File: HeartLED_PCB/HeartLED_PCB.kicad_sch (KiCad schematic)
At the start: 35 parts, among them U1 ICM7555IBAZ-T, U2 CD4017BM96, U3 TPS61222DCKR, U4 HX SS12F44G4

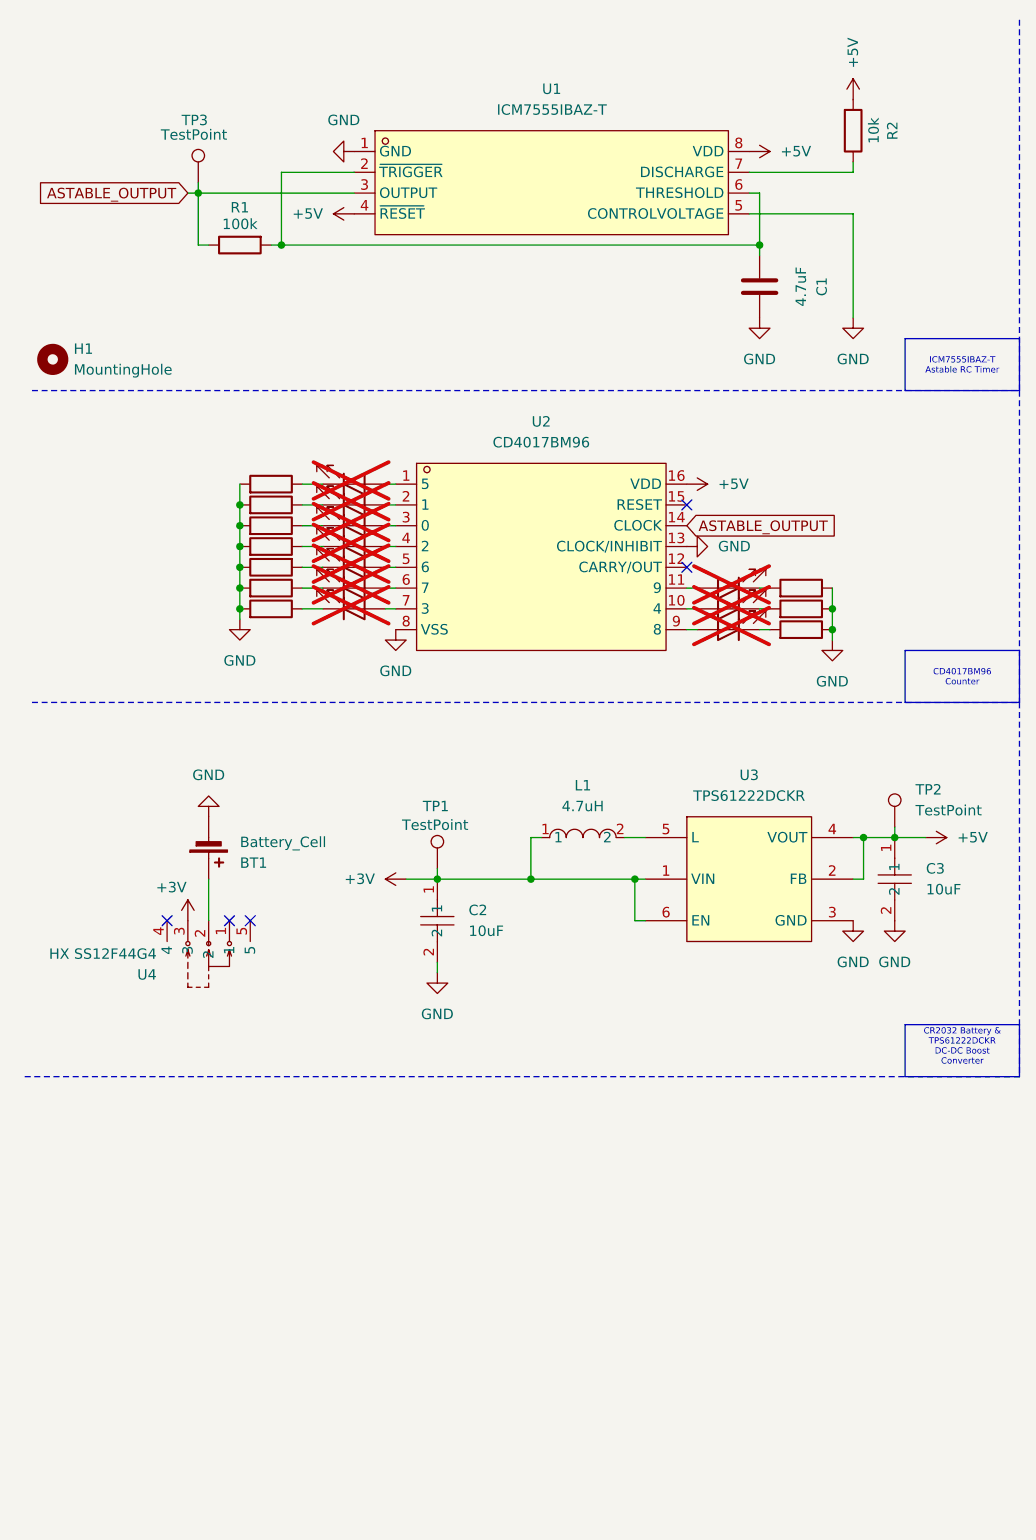
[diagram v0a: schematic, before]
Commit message: Ready to route
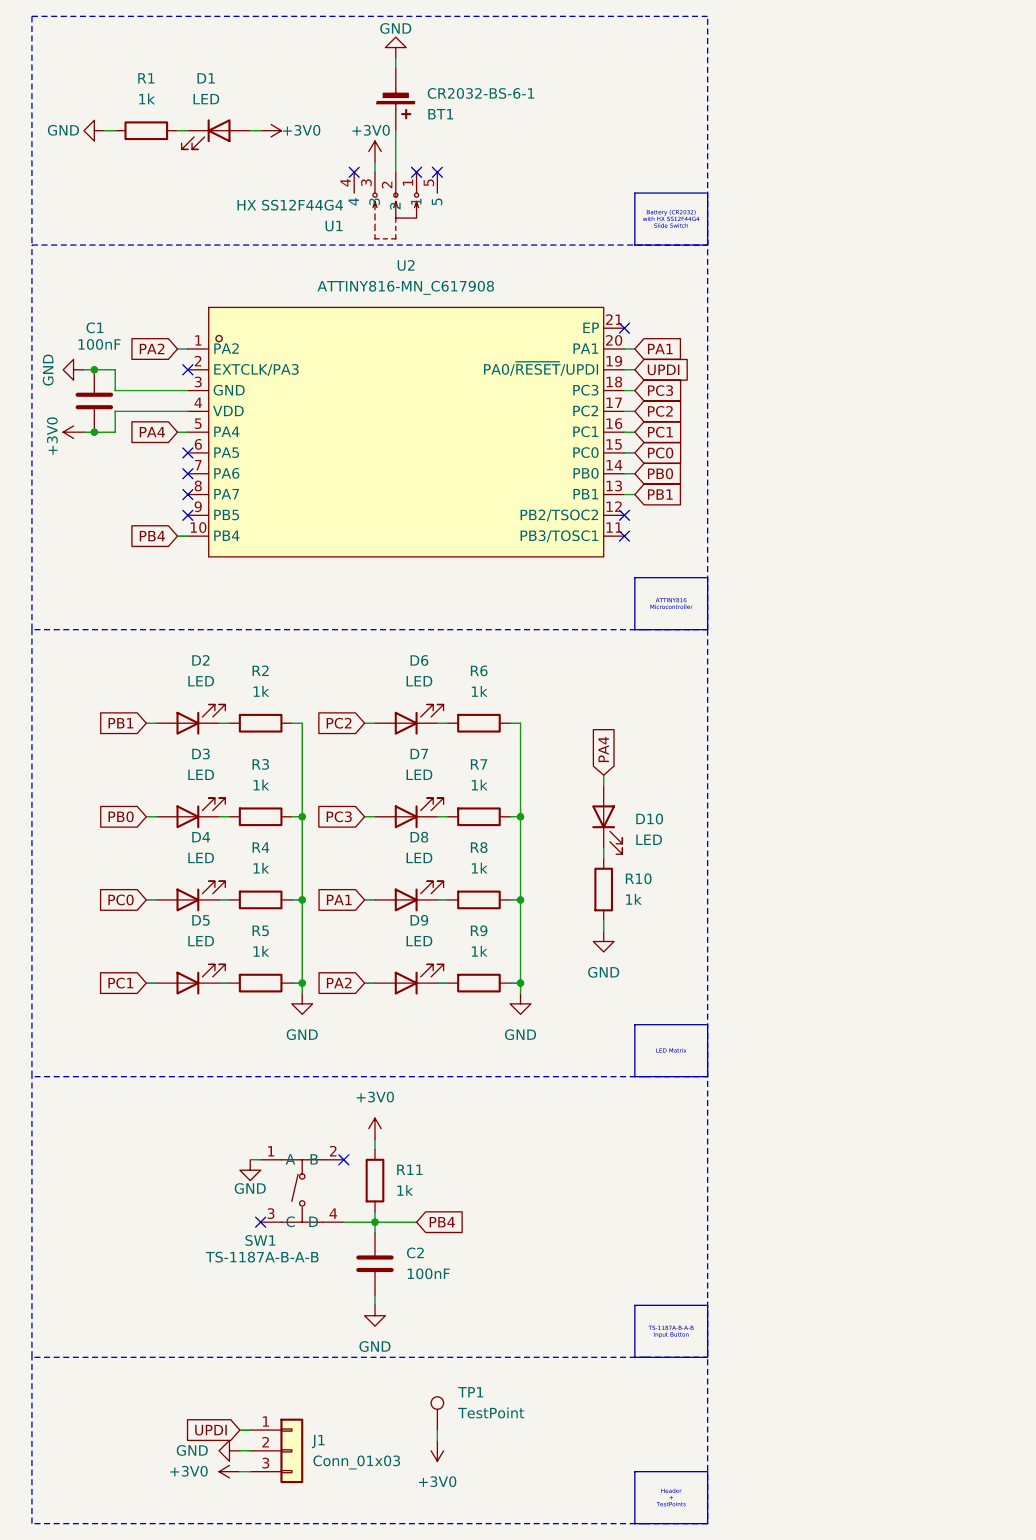
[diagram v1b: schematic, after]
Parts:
- removed C2, C3: 10uF, FOOTPRINTS:CL10A106MQ8NNNC, symbol CL10A106MQ8NNNC:CL10A106MQ8NNNC
- removed H1: MountingHole, MountingHole:MountingHole_2.1mm, symbol Mechanical:MountingHole
- removed L1: 4.7uH, FOOTPRINTS:LQH3NPN4R7MMEL, symbol LQH3NPN4R7MMEL:LQH3NPN4R7MMEL
- removed R12: 3.3k, FOOTPRINTS:0402WGJ0332TCE, symbol Device:R
- removed TP2, TP3: TestPoint, TestPoint:TestPoint_Pad_D1.0mm, symbol Connector:TestPoint
- removed U1: ICM7555IBAZ-T, FOOTPRINTS:ICM7555IBAZ-T, symbol ICM7555IBAZ-T:ICM7555IBAZ-T
- removed U2: CD4017BM96, FOOTPRINTS:CD4017BM96, symbol CD4017BM96:CD4017BM96
- removed U3: TPS61222DCKR, FOOTPRINTS:TPS61222DCKR, symbol TPS61222DCKR:TPS61222DCKR
- added C2: 100nF, FOOTPRINTS:0201X104K100CT, symbol Device:C
- added J1: Conn_01x03, Connector_PinHeader_2.54mm:PinHeader_1x03_P2.54mm_Vertical, symbol Connector_Generic:Conn_01x03
- added SW1: TS-1187A-B-A-B, FOOTPRINTS:TS-1187A-B-A-B, symbol TS-1187A-B-A-B:TS-1187A-B-A-B
- added U2: ATTINY816-MN_C617908, FOOTPRINTS:ATTINY816-MN, symbol ATTINY816-MN:ATTINY816-MN_C617908
- BT1: value Battery_Cell -> CR2032-BS-6-1; footprint Battery:BatteryHolder_Keystone_1060_1x2032 -> FOOTPRINTS:CR2032-BS-6-1; LCSC C5370859 -> C70377
- C1: value 4.7uF -> 100nF; footprint FOOTPRINTS:CL10A475KP8NNNC -> FOOTPRINTS:0201X104K100CT; LCSC C1705 -> C301918
- D1: footprint LED_THT:LED_D3.0mm -> FOOTPRINTS:F.0603.00026_P2-0603B1TS2-06T-001; LCSC (none) -> C7496819; now fitted
- D10, D2, D3, D4, D5, D6, D7, D8, D9: footprint LED_THT:LED_D3.0mm -> FOOTPRINTS:F.0603.00139_P2-0603R1TS2-06T-002; LCSC (none) -> C7496820; now fitted
- R1: value 100k -> 1k; footprint FOOTPRINTS:0603WAJ0104T5E -> FOOTPRINTS:0402WGJ0102TCE; LCSC C15458 -> C25543
- R10, R11, R3, R4, R5, R6, R7, R8, R9: value 3.3k -> 1k; footprint FOOTPRINTS:0402WGJ0332TCE -> FOOTPRINTS:0402WGJ0102TCE; LCSC C25936 -> C25543
- R2: value 10k -> 1k; footprint FOOTPRINTS:0402WGJ0103TCE -> FOOTPRINTS:0402WGJ0102TCE; LCSC C25531 -> C25543
- TP1: footprint TestPoint:TestPoint_Pad_D1.0mm -> TestPoint:TestPoint_Pad_D1.5mm
- renumbered U4 to U1
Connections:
- net +3V is gone; now on net +3V0: TP1.1, U1.3
- net +5V is gone; now on an unnamed net: R2.2
- net ASTABLE_OUTPUT is gone; now on net GND: R1.1
- net GND: now also C1.1, R10.2, R2.1, R3.1, R4.1, R5.1, R6.1, R8.1, R9.1, C2.2, J1.2 (Pin_2), SW1.1 (A), U2.3 (GND); no longer C1.2, R10.1, R11.1, R3.2, R4.2, R5.2, R6.2, R8.2, R9.2
- net +3V0: now reaches D1.2 (A)
- net +3V0: now also C1.2, R11.1, J1.3 (Pin_3), U2.4 (VDD)
- net PA2: now reaches D9.2 (A)
- net PA2: now also U2.1 (PA2)
- net PA4: now reaches D10.2 (A)
- net PA4: now also U2.5 (PA4)
- net PB1: now reaches D2.2 (A)
- net PB1: now also U2.13 (PB1)
- net PB0: now reaches D3.2 (A)
- net PB0: now also U2.14 (PB0)
- net PC0: now reaches D4.2 (A)
- net PC0: now also U2.15 (PC0)
- net PC1: now reaches D5.2 (A)
- net PC1: now also U2.16 (PC1)
- net PC2: now reaches D6.2 (A)
- net PC2: now also U2.17 (PC2)
- net PC3: now reaches D7.2 (A)
- net PC3: now also U2.18 (PC3)
- net PA1: now reaches D8.2 (A)
- net PA1: now also U2.20 (PA1)
- net at D6.1 (K): now also R6.2; no longer R8.1
- net at D1.1 (K): now also R1.2; no longer R3.1
- net at D8.1 (K): now also R8.2; no longer R10.2
- net at D3.1 (K): now also R3.2; no longer R5.1
- net at D10.1 (K): now also R10.1
- net at D9.1 (K): now also R9.2; no longer R11.2
- net at D5.1 (K): now also R5.2; no longer R7.2
- net at D2.1 (K): no longer R4.1
- net at D4.1 (K): now also R4.2; no longer R6.1
- net at D7.1 (K): now also R7.2; no longer R9.1
- new net PB4: C2.1, R11.2, SW1.4 (D), U2.10 (PB4)
- new net UPDI: J1.1 (Pin_1), U2.19 (PA0/~{RESET}/UPDI)
- no-connect marks 5 -> 13
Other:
- moved on the sheet: BT1, U1
